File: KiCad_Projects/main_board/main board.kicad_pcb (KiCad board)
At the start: 2 copper layers, 110 x 110 mm, 77 parts, among them J1 Conn_01x04_Female, J2 Conn_01x04_Female, J3 Conn_01x02_Female, J4 Conn_01x05_Female, SW1 SW_Push, SW2 SW_Push, U1 open_mv, U10 Seeeduino_Xiao, U11 Seeeduino_Xiao, U12 TSSP58038, U13 TSSP58038, U14 TSSP58038, U15 TSSP58038, U2 type-c_sirial, U3 PIC18F26K20_ISS, U4 Akizuki_Logiv_Level_converter, U5 MPU6050, U6 TSSP58038, U7 TSSP58038, U8 TSSP58038, U9 TSSP58038

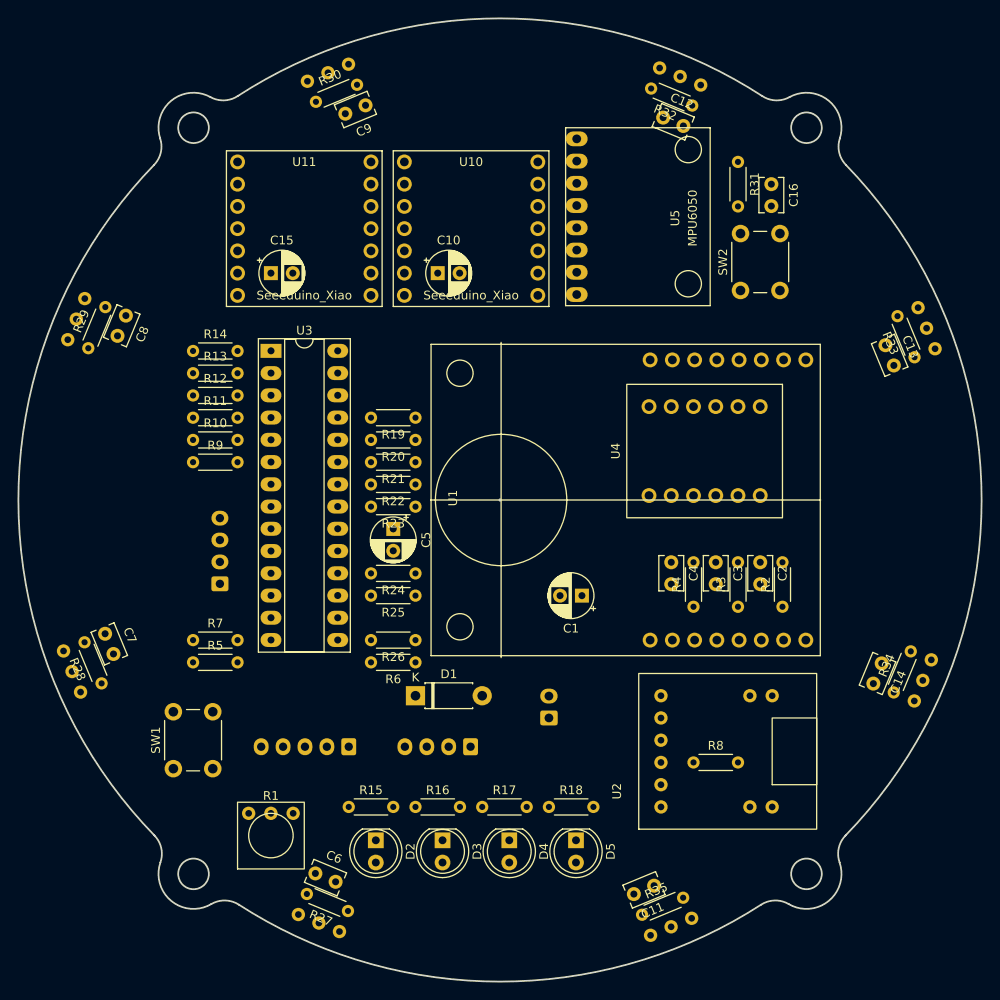
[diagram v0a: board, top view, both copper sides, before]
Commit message: 基板データの更新
最後に更新してからのデータ全てです。
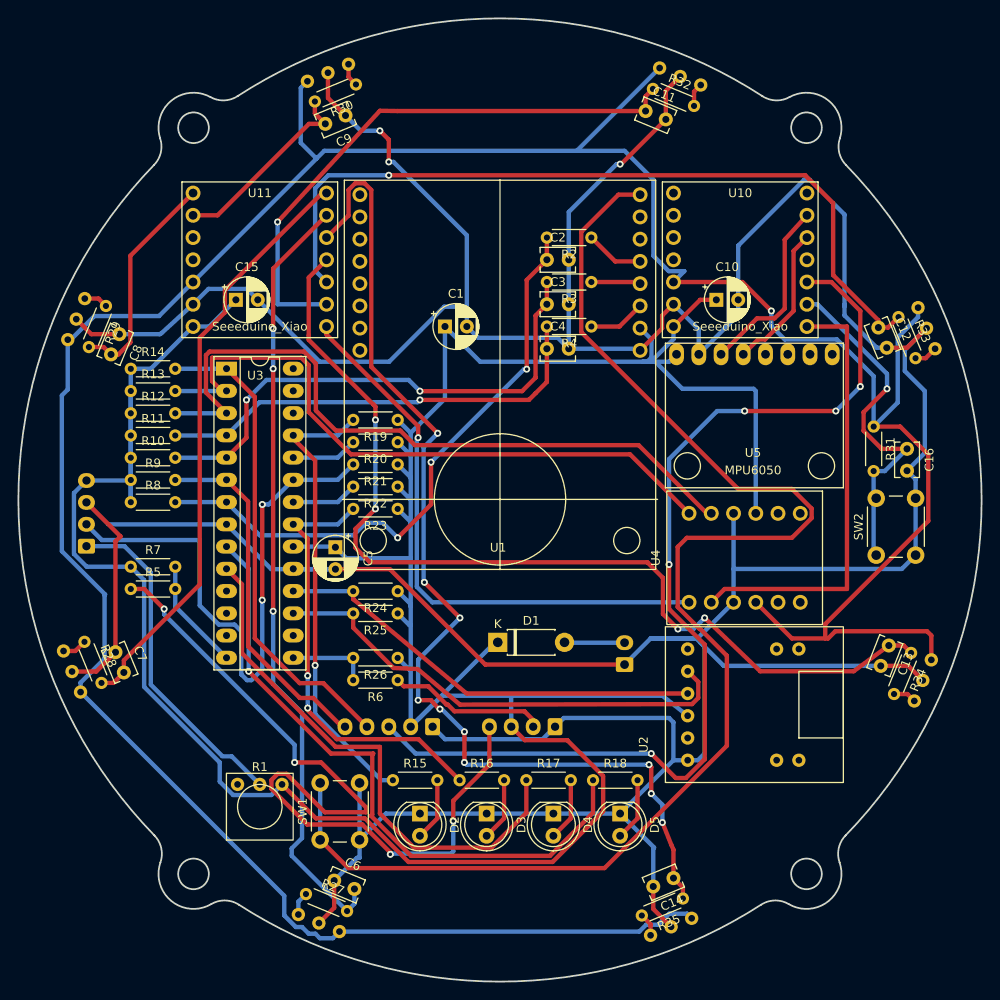
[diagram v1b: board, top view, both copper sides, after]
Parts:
- moved C11 88.5 mm to (117.7, 72.9), turned to -22.5 degrees
- moved R8 70.8 mm to (58.9, 117.6)
- moved R2 47.5 mm to (111.5, 87.4), turned to 180 degrees
- moved C2 42.3 mm to (106.4, 89.9), turned to 0 degrees
- moved R3 40.7 mm to (111.5, 92.5), turned to 180 degrees
- moved C3 35.2 mm to (106.4, 95.0), turned to 0 degrees
- moved C1 34.5 mm to (94.8, 97.5), turned to 0 degrees
- moved C12 34.3 mm to (144.3, 97.7), turned to -67.5 degrees
- moved C13 34.3 mm to (145.5, 134.0), turned to -111.5 degrees
- moved C14 34.2 mm to (120.9, 160.5), turned to -157.5 degrees
- moved R4 34.1 mm to (111.5, 97.5), turned to 180 degrees
- moved C16 34.0 mm to (147.6, 111.5)
- moved R31 34.0 mm to (143.8, 109.0)
- moved SW2 34.0 mm to (144.1, 123.6)
- moved C10 32.0 mm to (125.8, 94.5)
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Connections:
- C1 pad 2: RES -> GND
- C10 pad 2: RES -> GND
- C11 pad 1: RES -> IR1
- C11 pad 2: +3V3 -> GND
- C12 pad 1: RES -> IR2
- C12 pad 2: +3V3 -> GND
- C13 pad 1: RES -> IR3
- C13 pad 2: +3V3 -> GND
- C14 pad 1: RES -> IR4
- C14 pad 2: +3V3 -> GND
- C15 pad 2: RES -> GND
- C16 pad 1: Net-(C16-Pad1) -> RES
- C16 pad 2: RES -> GND
- C2 pad 2: RES -> GND
- C3 pad 2: RES -> GND
- C4 pad 2: RES -> GND
- C5 pad 2: RES -> GND
- C6 pad 1: +3V3 -> GND
- C6 pad 2: RES -> IR5
- C7 pad 1: +3V3 -> GND
- C7 pad 2: RES -> IR6
- C8 pad 1: +3V3 -> GND
- C8 pad 2: RES -> IR7
- C9 pad 1: +3V3 -> GND
- C9 pad 2: RES -> IR8
- D2 pad 1: RES -> GND
- D3 pad 1: RES -> GND
- D4 pad 1: RES -> GND
- D5 pad 1: RES -> GND
- J1 pad 1: RES -> GND
- J2 pad 3: RES -> GND
- J3 pad 1: RES -> GND
- J4 pad 1: RES -> GND
- R27 pad 1: Net-(R27-Pad1) -> Net-(U6-Pad0)
- R27 pad 2: +3V3 -> IR5
- R28 pad 1: Net-(R28-Pad1) -> Net-(U7-Pad0)
- R28 pad 2: +3V3 -> IR6
- R29 pad 1: Net-(R29-Pad1) -> Net-(U8-Pad0)
- R29 pad 2: +3V3 -> IR7
- R30 pad 1: Net-(R30-Pad1) -> Net-(U9-Pad0)
- R30 pad 2: +3V3 -> IR8
- R31 pad 2: Net-(C16-Pad1) -> RES
- R32 pad 1: +3V3 -> IR1
- R32 pad 2: Net-(R32-Pad2) -> Net-(U12-Pad0)
- R33 pad 1: +3V3 -> IR2
- R33 pad 2: Net-(R33-Pad2) -> Net-(U13-Pad0)
- R34 pad 1: +3V3 -> IR3
- R34 pad 2: Net-(R34-Pad2) -> Net-(U14-Pad0)
- R35 pad 1: +3V3 -> IR4
- R35 pad 2: Net-(R35-Pad2) -> Net-(U15-Pad0)
- SW1 pad 2: RES -> GND
- SW2 pad 1: Net-(C16-Pad1) -> RES
- SW2 pad 2: RES -> GND
- U1 pad 9: RES -> GND
- U10 pad 13: RES -> GND
- U11 pad 13: RES -> GND
- U12 pad 0: IR1 -> Net-(U12-Pad0)
- U12 pad 1: RES -> GND
- U12 pad 2: Net-(R32-Pad2) -> +3V3
- U13 pad 0: IR2 -> Net-(U13-Pad0)
- U13 pad 1: RES -> GND
- U13 pad 2: Net-(R33-Pad2) -> +3V3
- U14 pad 0: IR3 -> Net-(U14-Pad0)
- U14 pad 1: RES -> GND
- U14 pad 2: Net-(R34-Pad2) -> +3V3
- U15 pad 0: IR4 -> Net-(U15-Pad0)
- U15 pad 1: RES -> GND
- U15 pad 2: Net-(R35-Pad2) -> +3V3
- U2 pad 1: RES -> GND
- U3 pad 19: RES -> GND
- U3 pad 8: RES -> GND
- U4 pad 10: RES -> GND
- U4 pad 3: RES -> GND
- U5 pad 2: RES -> GND
- U6 pad 0: IR5 -> Net-(U6-Pad0)
- U6 pad 1: RES -> GND
- U6 pad 2: Net-(R27-Pad1) -> +3V3
- U7 pad 0: IR6 -> Net-(U7-Pad0)
- U7 pad 1: RES -> GND
- U7 pad 2: Net-(R28-Pad1) -> +3V3
- U8 pad 0: IR7 -> Net-(U8-Pad0)
- U8 pad 1: RES -> GND
- U8 pad 2: Net-(R29-Pad1) -> +3V3
- U9 pad 0: IR8 -> Net-(U9-Pad0)
- U9 pad 1: RES -> GND
- U9 pad 2: Net-(R30-Pad1) -> +3V3
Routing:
- net GND: track 0.00 -> 548.2 mm, vias 0 -> 3
- net +5V: track 0.00 -> 362.1 mm
- net +3V3: track 0.00 -> 351.3 mm, vias 0 -> 1
- net Net-(SW1-Pad1): track 0.00 -> 157.5 mm
- net IR4: track 0.00 -> 123.8 mm, vias 0 -> 10
- net SW2: track 0.00 -> 116.7 mm, vias 0 -> 5
- net IR3: track 0.00 -> 111.8 mm, vias 0 -> 4
- net Net-(J1-Pad4): track 0.00 -> 93.3 mm, vias 0 -> 4
- net IR2: track 0.00 -> 91.5 mm, vias 0 -> 1
- net IR5: track 0.00 -> 89.3 mm, vias 0 -> 3
- net AD2: track 0.00 -> 82.1 mm
- net AD1: track 0.00 -> 75.6 mm
- net PWR LED: track 0.00 -> 73.6 mm, vias 0 -> 1
- net AD5: track 0.00 -> 69.8 mm, vias 0 -> 3
- net IR6: track 0.00 -> 67.7 mm
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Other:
- outline, holes or cut-outs redrawn
